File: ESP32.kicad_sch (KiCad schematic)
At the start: 30 parts, among them J201 GPIO, J202 Power, J203 Conn_01x01, J206 IO, J207 Conn_01x07, U201 ESP32-WROOM-32E

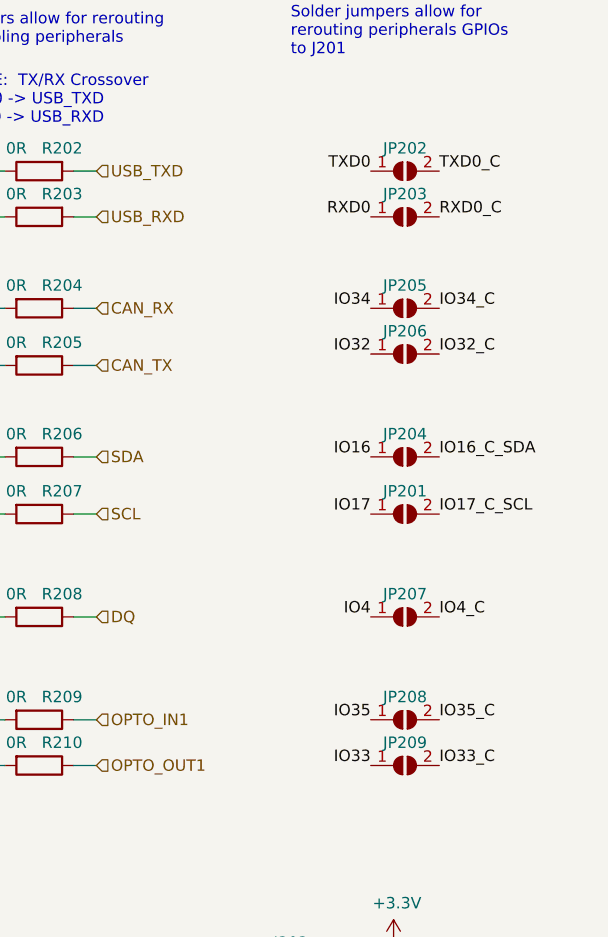
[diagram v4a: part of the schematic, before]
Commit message: Save schema with KiCad 7.0.6
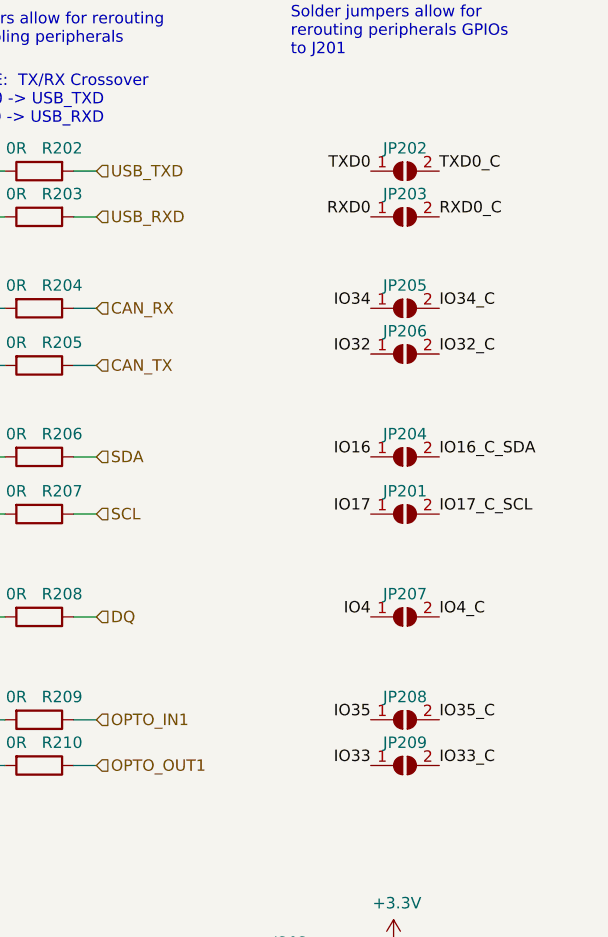
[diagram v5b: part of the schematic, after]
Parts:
- U201: JLCPCB_CORRECTION (none) -> 0;-2.25;270

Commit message: Update BAT54AW part # for availability
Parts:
- D1101, D1102: LCSC C78261 -> C134404
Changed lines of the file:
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@@
       (effects (font (size 1.27 1.27)) hide)
     )
-    (property "LCSC" "C78261" (at 46.99 139.7 90)
+    (property "LCSC" "C134404" (at 46.99 139.7 90)
       (effects (font (size 1.27 1.27)) hide)
     )
@@
       (effects (font (size 1.27 1.27)) hide)
     )
-    (property "LCSC" "C78261" (at 46.99 171.45 90)
+    (property "LCSC" "C134404" (at 46.99 171.45 90)
       (effects (font (size 1.27 1.27)) hide)
     )

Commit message: Fix component rotations
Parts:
- D1101, D1102: JLCPCB_CORRECTION (none) -> 0;0;180
- J201: JLCPCB_CORRECTION (none) -> 1.27;24.13;90
- J202: JLCPCB_CORRECTION (none) -> 1.27;2.54;90
- U201: JLCPCB_CORRECTION 0;-2.25;270 -> 0;0.8;270
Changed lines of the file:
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@@
       (effects (font (size 1.27 1.27)) hide)
     )
-    (property "JLCPCB_CORRECTION" "" (at 138.43 66.04 0)
+    (property "JLCPCB_CORRECTION" "1.27;24.13;90" (at 138.43 66.04 0)
       (effects (font (size 1.27 1.27)) hide)
     )
@@
       (effects (font (size 1.27 1.27)) hide)
     )
-    (property "JLCPCB_CORRECTION" "" (at 237.49 132.715 0)
+    (property "JLCPCB_CORRECTION" "1.27;2.54;90" (at 237.49 132.715 0)
       (effects (font (size 1.27 1.27)) hide)
     )
@@
       (effects (font (size 1.27 1.27)) hide)
     )
-    (property "JLCPCB_CORRECTION" "0;-2.25;270" (at 64.77 73.66 0)
+    (property "JLCPCB_CORRECTION" "0;0.8;270" (at 64.77 73.66 0)
       (effects (font (size 1.27 1.27)) hide)
     )
@@
       (effects (font (size 1.27 1.27)) hide)
     )
-    (property "JLCPCB_CORRECTION" "" (at 46.99 139.7 0)
+    (property "JLCPCB_CORRECTION" "0;0;180" (at 46.99 139.7 0)
       (effects (font (size 1.27 1.27)) hide)
     )
@@
       (effects (font (size 1.27 1.27)) hide)
     )
-    (property "JLCPCB_CORRECTION" "" (at 46.99 171.45 0)
-      (effects (font (size 1.27 1.27)) hide)
-    )
+    (property "JLCPCB_CORRECTION" "0;0;180" (at 46.99 171.45 0)
+      (effects (font (size 1.27 1.27)) hide)
+    )
